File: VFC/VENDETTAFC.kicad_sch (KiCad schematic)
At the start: 16 parts, among them U1 STM32F722RETx, Y3 C3E-8.000-18-3030-X-R

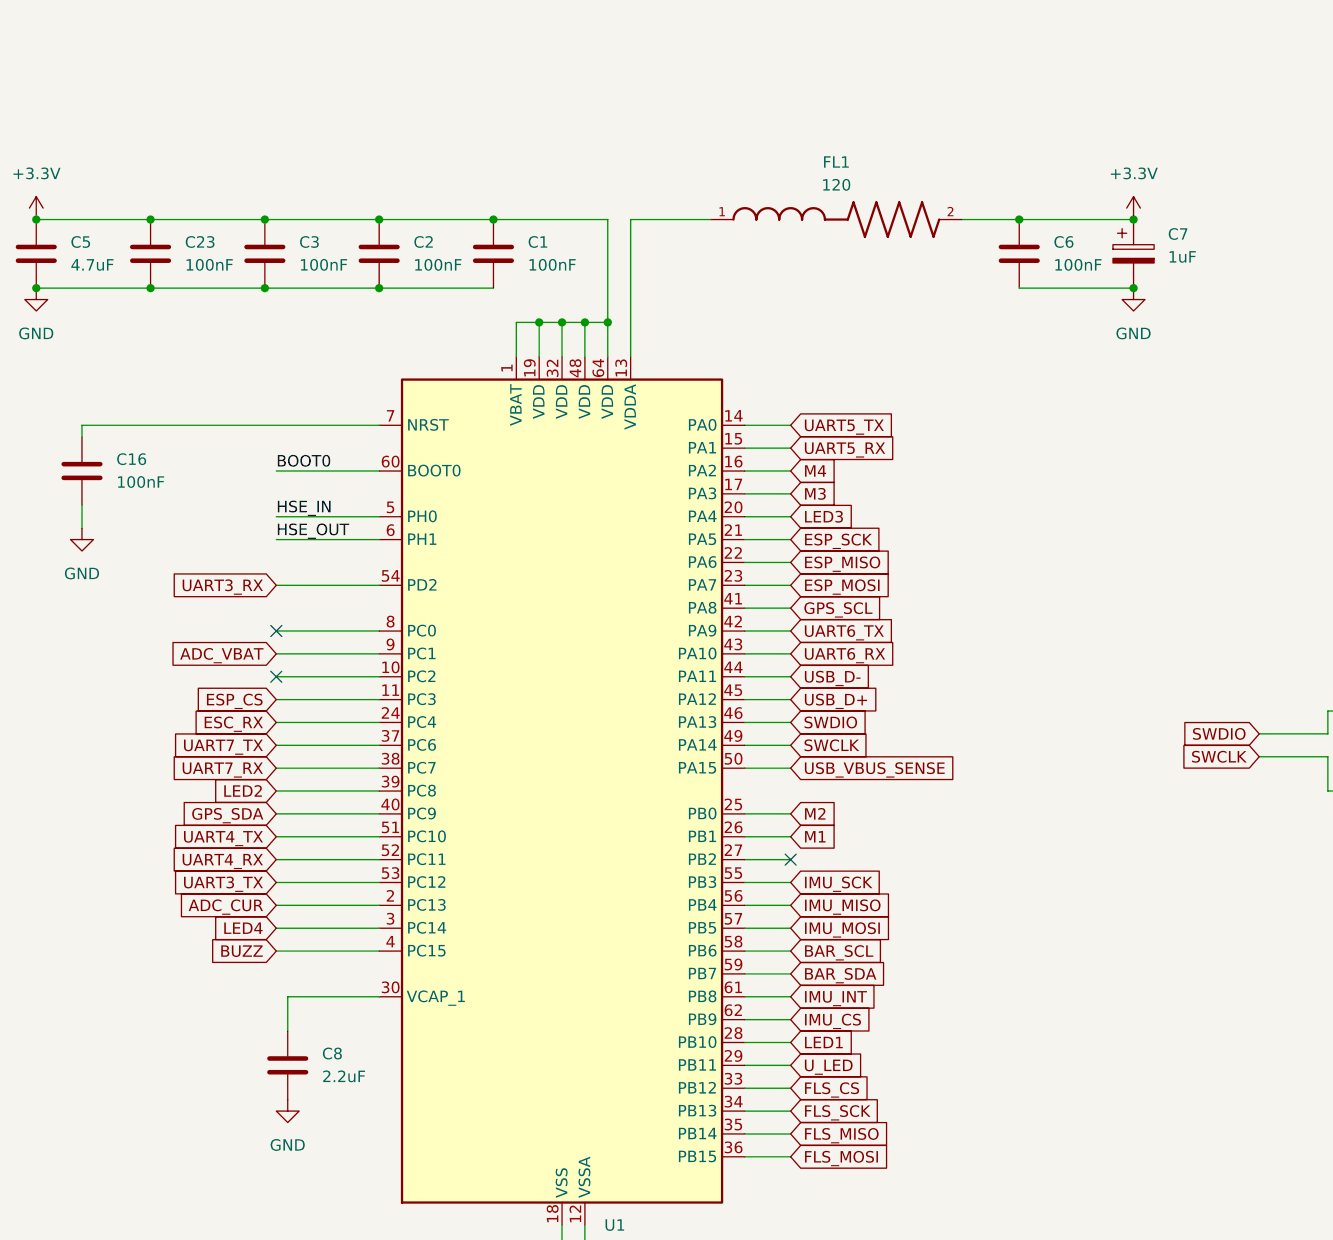
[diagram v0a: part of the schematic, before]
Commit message: VFC PCB traces update
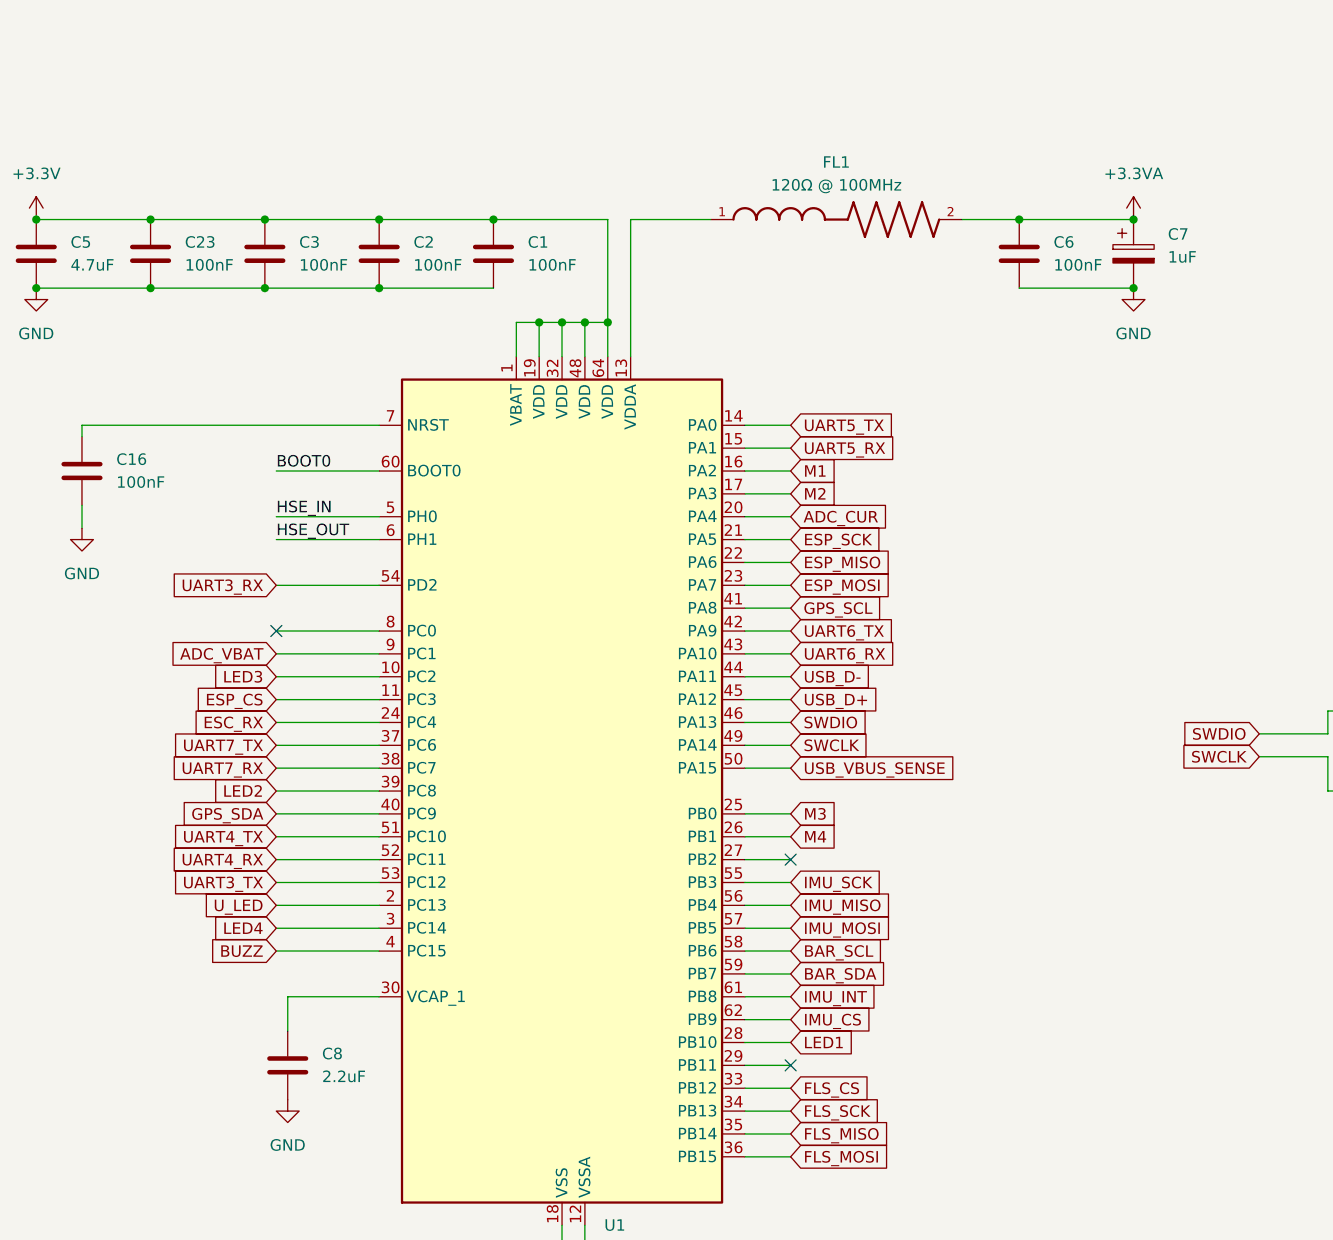
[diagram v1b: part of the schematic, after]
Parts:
- FL1: value 120 -> 120Ω @ 100MHz
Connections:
- net +3.3V: no longer C6.1, C7.1, FL1.2
- net ADC_CUR: now also U1.20 (PA4); no longer U1.2 (PC13)
- net LED3: now also U1.10 (PC2); no longer U1.20 (PA4)
- net M1: now also U1.16 (PA2); no longer U1.26 (PB1)
- net M2: now also U1.17 (PA3); no longer U1.25 (PB0)
- net M3: now also U1.25 (PB0); no longer U1.17 (PA3)
- net M4: now also U1.26 (PB1); no longer U1.16 (PA2)
- net U_LED: now also U1.2 (PC13); no longer U1.29 (PB11)
- new net +3.3VA: C6.1, C7.1, FL1.2
